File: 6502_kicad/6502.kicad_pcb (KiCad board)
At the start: 2 copper layers, 82.5 x 133.4 mm, 19 parts, among them J1 Conn_01x02, J2 Conn_02x10_Odd_Even, J3 Conn_02x10_Odd_Even, J4 Conn_01x08, U1 24LC256, U10 74HC04, U13 W65C51N, U14 74LS138, U15 WD65C22, U16 WD65C22, U2 74HC595, U3 WD65C02, U4 628128, U5 74HC595, U6 ATmega328P-PU, U7 74LS30, U8 74HC595, U9 74LS08

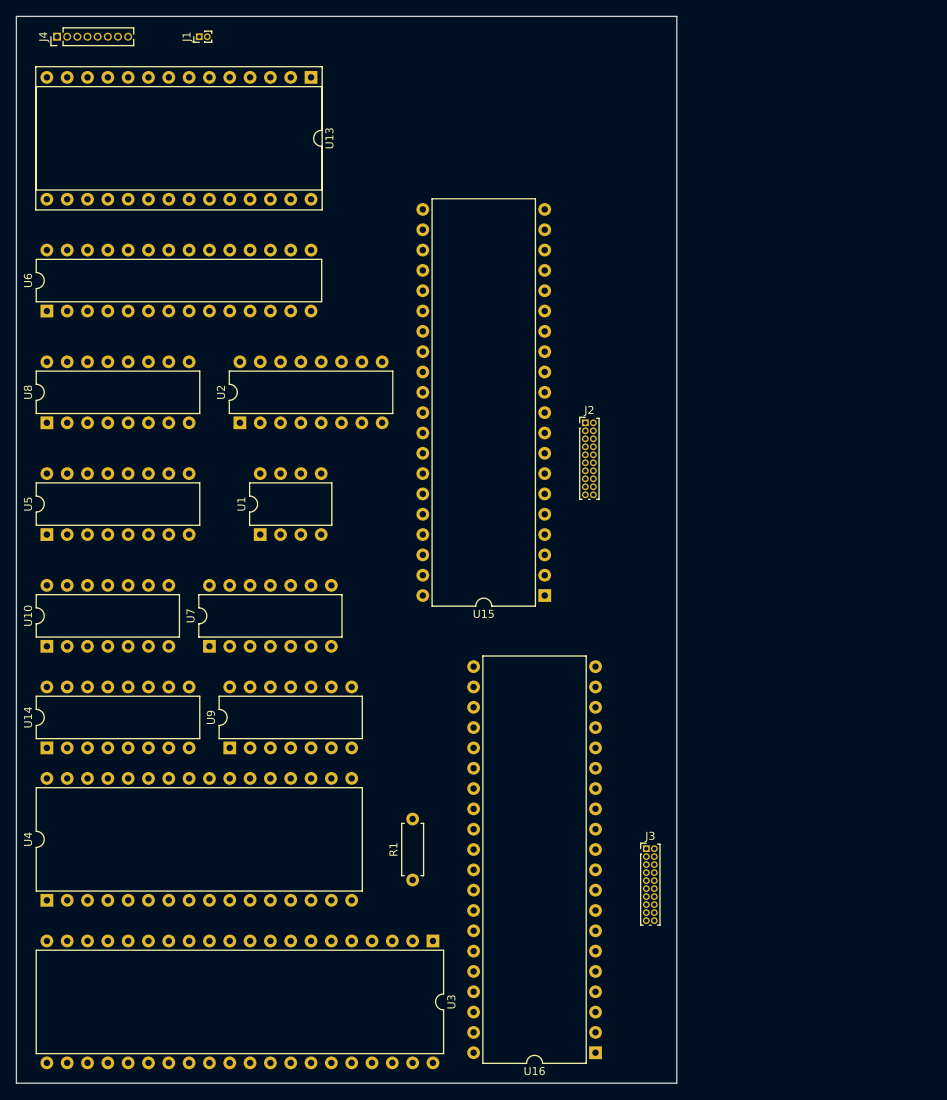
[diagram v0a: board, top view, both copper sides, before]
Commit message: Working on kicad.
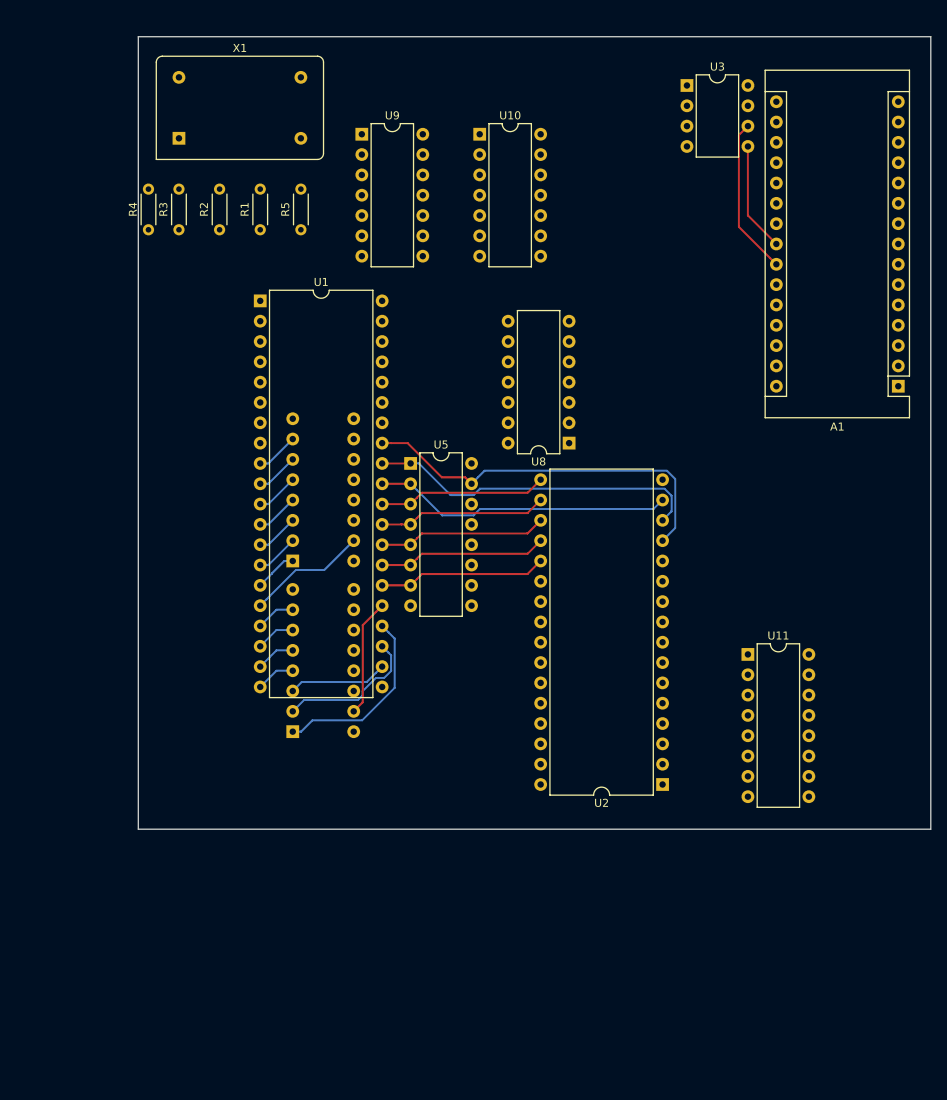
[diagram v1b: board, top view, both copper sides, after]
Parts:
- removed J1: Conn_01x02, Connector_PinHeader_1.00mm:PinHeader_1x02_P1.00mm_Vertical
- removed J2, J3: Conn_02x10_Odd_Even, Connector_PinHeader_1.00mm:PinHeader_2x10_P1.00mm_Vertical
- removed J4: Conn_01x08, Connector_PinHeader_1.27mm:PinHeader_1x08_P1.27mm_Vertical
- removed U13: W65C51N, Package_DIP:DIP-28_W15.24mm_Socket
- removed U14: 74LS138, Package_DIP:DIP-16_W7.62mm
- removed U15, U16: WD65C22, Package_DIP:DIP-40_W15.24mm
- removed U4: 628128, Package_DIP:DIP-32_W15.24mm
- added A1: Arduino_Nano_v2.x, Module:Arduino_Nano, F.Cu at (122.9, 58.9)
- added R2: 3.3K, Resistor_THT:R_Axial_DIN0204_L3.6mm_D1.6mm_P5.08mm_Horizontal, F.Cu at (38.1, 39.4)
- added R3: 3.3K, Resistor_THT:R_Axial_DIN0204_L3.6mm_D1.6mm_P5.08mm_Horizontal, F.Cu at (33.0, 39.4)
- added R4: 3.3K, Resistor_THT:R_Axial_DIN0204_L3.6mm_D1.6mm_P5.08mm_Horizontal, F.Cu at (29.2, 39.4)
- added R5: 3.3K, Resistor_THT:R_Axial_DIN0204_L3.6mm_D1.6mm_P5.08mm_Horizontal, F.Cu at (48.3, 39.4)
- added U11: 74LS138, Package_DIP:DIP-16_W7.62mm, F.Cu at (104.1, 92.5)
- added X1: CXO_DIP14, Oscillator:Oscillator_DIP-14, F.Cu at (33.0, 27.9)
- R1: value 1K -> 3.3K; footprint Resistor_THT:R_Axial_DIN0207_L6.3mm_D2.5mm_P7.62mm_Horizontal -> Resistor_THT:R_Axial_DIN0204_L3.6mm_D1.6mm_P5.08mm_Horizontal
- U1: value 24LC256 -> WD65C02; footprint Package_DIP:DIP-8_W7.62mm -> Package_DIP:DIP-40_W15.24mm
- U10: value 74HC04 -> 74LS04
- U2: value 74HC595 -> 628128; footprint Package_DIP:DIP-16_W7.62mm -> Package_DIP:DIP-32_W15.24mm
- U3: value WD65C02 -> 24C256; footprint Package_DIP:DIP-40_W15.24mm -> Package_DIP:DIP-8_W7.62mm
- U5: value 74HC595 -> 74HCT595
- U6: value ATmega328P-PU -> 74HCT595; footprint Package_DIP:DIP-28_W7.62mm -> Package_DIP:DIP-16_W7.62mm; moved to B.Cu
- U7: value 74LS30 -> 74HCT595; footprint Package_DIP:DIP-14_W7.62mm -> Package_DIP:DIP-16_W7.62mm; moved to B.Cu
- U8: value 74HC595 -> 74LS30; footprint Package_DIP:DIP-16_W7.62mm -> Package_DIP:DIP-14_W7.62mm
- moved U3 111.5 mm to (96.5, 21.3), turned to 0 degrees
- moved U10 83.8 mm to (70.6, 27.4), turned to 0 degrees
- moved R1 83.5 mm to (43.2, 39.4)
- moved U9 78.5 mm to (55.9, 27.4), turned to 0 degrees
- moved U2 69.5 mm to (93.5, 108.7), turned to 180 degrees
- moved U8 65.3 mm to (81.8, 66.0), turned to 180 degrees
- moved U5 46.3 mm to (62.0, 68.6), turned to 0 degrees
- moved U6 43.8 mm to (47.2, 80.8), turned to 0 degrees
- moved U1 29.2 mm to (43.2, 48.3), turned to 0 degrees
- moved U7 14.9 mm to (47.2, 102.1), turned to 0 degrees
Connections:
- U1 pad 2: Net-(U1-Pad1) -> Net-(R2-Pad1)
- U1 pad 3: Net-(U1-Pad1) -> Net-(U1-Pad3)
- U1 pad 6: Net-(U1-Pad6) -> Net-(R4-Pad1)
- U1 pad 8: Net-(U1-Pad8) -> +5V
- U10 pad 1: Net-(U10-Pad1) -> /a7
- U10 pad 10: (no net) -> Net-(U10-Pad10)
- U10 pad 11: (no net) -> Net-(U10-Pad11)
- U10 pad 12: (no net) -> Net-(U10-Pad12)
- U10 pad 13: (no net) -> Net-(U10-Pad13)
- U10 pad 3: /a7 -> Net-(U10-Pad3)
- U10 pad 5: Net-(U10-Pad5) -> /~CS_RAM
- U10 pad 6: Net-(U10-Pad6) -> /CS_IO
- U2 pad 1: /d6 -> (no net)
- U2 pad 10: Net-(U2-Pad10) -> /a2
- U2 pad 11: Net-(U2-Pad11) -> /a1
- U2 pad 12: Net-(U2-Pad10) -> /a0
- U2 pad 13: Net-(U2-Pad13) -> /d0
- U2 pad 14: Net-(U2-Pad14) -> /d1
- U2 pad 15: /d7 -> /d2
- U2 pad 16: Net-(U2-Pad10) -> GND
- U2 pad 2: /d5 -> GND
- U2 pad 3: /d4 -> /a14
- U2 pad 4: /d3 -> /a12
- U2 pad 5: /d2 -> /a7
- U2 pad 6: /d1 -> /a6
- U2 pad 7: /d0 -> /a5
- U2 pad 8: Net-(U1-Pad1) -> /a4
- U2 pad 9: Net-(U2-Pad9) -> /a3
- U3 pad 1: Net-(U3-Pad1) -> GND
- U3 pad 2: Net-(R1-Pad1) -> GND
- U3 pad 3: Net-(U3-Pad3) -> GND
- U3 pad 4: Net-(U15-Pad21) -> GND
- U3 pad 7: Net-(U3-Pad7) -> +5V
- U5 pad 1: /a6 -> /d1
- U5 pad 10: Net-(U2-Pad10) -> Net-(U5-Pad10)
- U5 pad 11: Net-(U2-Pad11) -> Net-(A1-Pad6)
- U5 pad 12: Net-(U2-Pad10) -> Net-(A1-Pad7)
- U5 pad 13: Net-(U2-Pad13) -> /Bus_Enable
- U5 pad 15: /a7 -> /d0
- U5 pad 16: Net-(U2-Pad10) -> +5V
- U5 pad 2: /a5 -> /d2
- U5 pad 3: /a4 -> /d3
- U5 pad 4: /a3 -> /d4
- U5 pad 5: /a2 -> /d5
- U5 pad 6: /a1 -> /d6
- U5 pad 7: /a0 -> /d7
- U5 pad 8: Net-(U1-Pad1) -> GND
- U5 pad 9: Net-(U2-Pad14) -> Net-(U5-Pad9)
- U6 pad 1: Net-(U6-Pad1) -> /a6
- U6 pad 11: /d5 -> Net-(A1-Pad6)
- U6 pad 12: /d6 -> Net-(A1-Pad7)
- U6 pad 13: /d7 -> /Bus_Enable
- U6 pad 14: /d0 -> Net-(U6-Pad14)
- U6 pad 15: /d1 -> /a7
- U6 pad 16: Net-(U6-Pad16) -> +5V
- U6 pad 2: Net-(U6-Pad2) -> /a5
- U6 pad 3: Net-(U6-Pad3) -> /a4
- U6 pad 4: /d2 -> /a3
- U6 pad 5: /d3 -> /a2
- U6 pad 6: /d4 -> /a1
- U6 pad 7: Net-(U6-Pad7) -> /a0
- U6 pad 8: Net-(U6-Pad22) -> GND
- U6 pad 9: Net-(U6-Pad9) -> Net-(U5-Pad14)
- U7 pad 1: /a15 -> /a14
- U7 pad 10: (no net) -> Net-(U7-Pad10)
- U7 pad 11: /a9 -> Net-(A1-Pad6)
- U7 pad 12: /a8 -> Net-(A1-Pad7)
- U7 pad 13: (no net) -> /Bus_Enable
- U7 pad 14: (no net) -> Net-(A1-Pad5)
- U7 pad 2: /a14 -> /a13
- U7 pad 3: /a13 -> /a12
- U7 pad 4: /a12 -> /a11
- U7 pad 5: /a11 -> /a10
- U7 pad 6: /a10 -> /a9
- U7 pad 7: (no net) -> /a8
- U7 pad 8: Net-(U10-Pad1) -> GND
- U7 pad 9: (no net) -> Net-(U6-Pad14)
- U8 pad 1: /a14 -> /a15
- U8 pad 10: Net-(U2-Pad10) -> (no net)
- U8 pad 11: Net-(U2-Pad11) -> /a9
- U8 pad 12: Net-(U2-Pad10) -> /a8
- U8 pad 13: Net-(U2-Pad13) -> (no net)
- U8 pad 14: Net-(U6-Pad26) -> (no net)
- U8 pad 2: /a13 -> /a14
- U8 pad 3: /a12 -> /a13
- U8 pad 4: /a11 -> /a12
- U8 pad 5: /a10 -> /a11
- U8 pad 6: /a9 -> /a10
- U8 pad 7: /a8 -> (no net)
- U8 pad 8: Net-(U8-Pad8) -> Net-(U10-Pad3)
- U8 pad 9: Net-(U5-Pad14) -> (no net)
- U9 pad 10: (no net) -> Net-(U9-Pad10)
- U9 pad 11: (no net) -> Net-(U9-Pad11)
- U9 pad 12: (no net) -> Net-(U9-Pad12)
- U9 pad 13: (no net) -> Net-(U9-Pad13)
- U9 pad 3: Net-(U10-Pad5) -> /~CS_RAM
- U9 pad 4: Net-(U10-Pad6) -> (no net)
- U9 pad 5: Net-(U15-Pad25) -> (no net)
- U9 pad 6: Net-(U4-Pad30) -> (no net)
- U9 pad 8: (no net) -> Net-(U9-Pad8)
- U9 pad 9: (no net) -> Net-(U9-Pad9)
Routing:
- net /d0: track 0.00 -> 48.2 mm
- net /d1: track 0.00 -> 42.1 mm
- net /d2: track 0.00 -> 37.5 mm
- net /a14: track 0.00 -> 23.4 mm
- net /d6: track 0.00 -> 21.1 mm
- net /d5: track 0.00 -> 21.1 mm
- net /d3: track 0.00 -> 21.1 mm
- net /d4: track 0.00 -> 21.1 mm
- net /d7: track 0.00 -> 21.1 mm
- net Net-(A1-Pad24): track 0.00 -> 19.7 mm
- net /a13: track 0.00 -> 18.2 mm
- net /a7: track 0.00 -> 15.1 mm
- net /a15: track 0.00 -> 14.7 mm
- net Net-(A1-Pad23): track 0.00 -> 13.7 mm
- net /a12: track 0.00 -> 12.4 mm
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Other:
- board size 82.5 x 133.4 mm -> 99.1 x 99.1 mm
